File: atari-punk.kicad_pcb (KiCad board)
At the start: 2 copper layers, 74.7 x 54.4 mm, 25 parts, among them J1 Barrel_Jack_Switch, J2 Euro_Power, J3 CV1_IN, J4 CV2_IN, J5 CV3_IN, J6 CV4_IN, J7 AUDIO_OUT, U1 LM555xN, U2 LM555xN

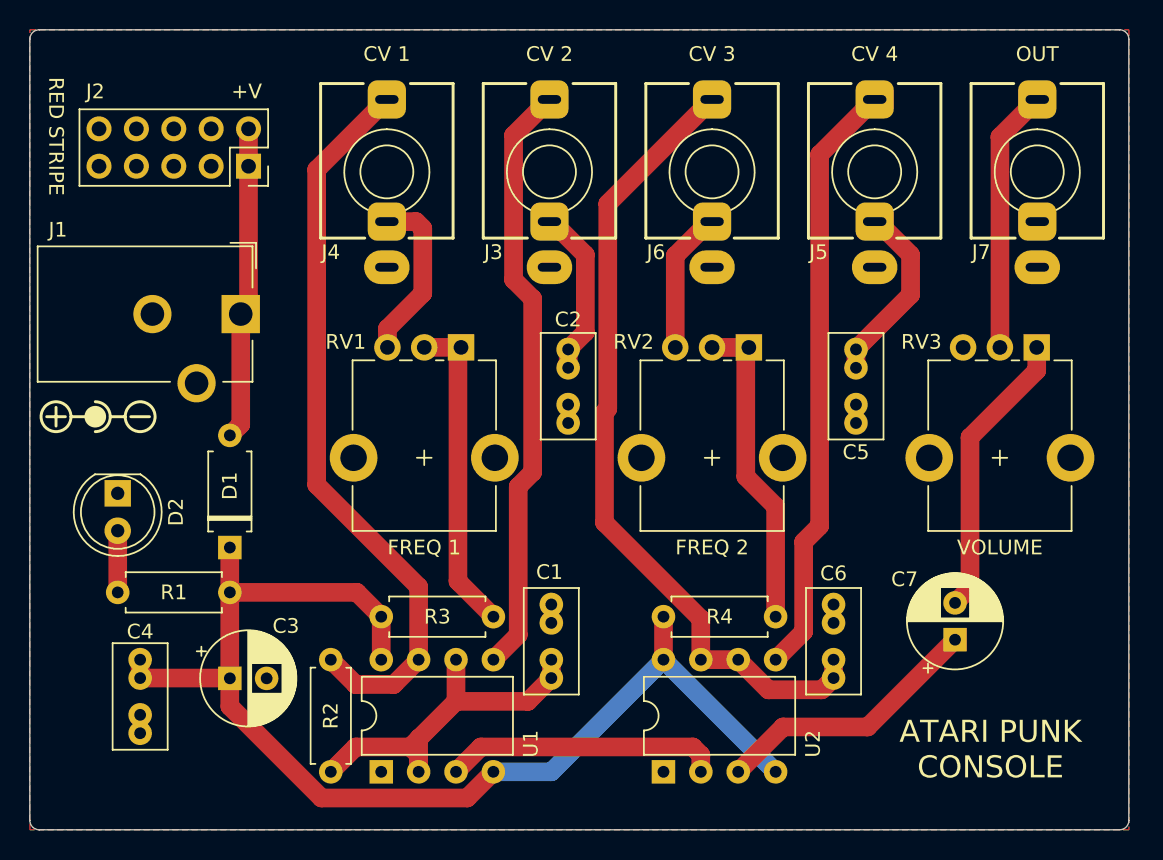
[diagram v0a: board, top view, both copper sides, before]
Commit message: Fixing for rev2
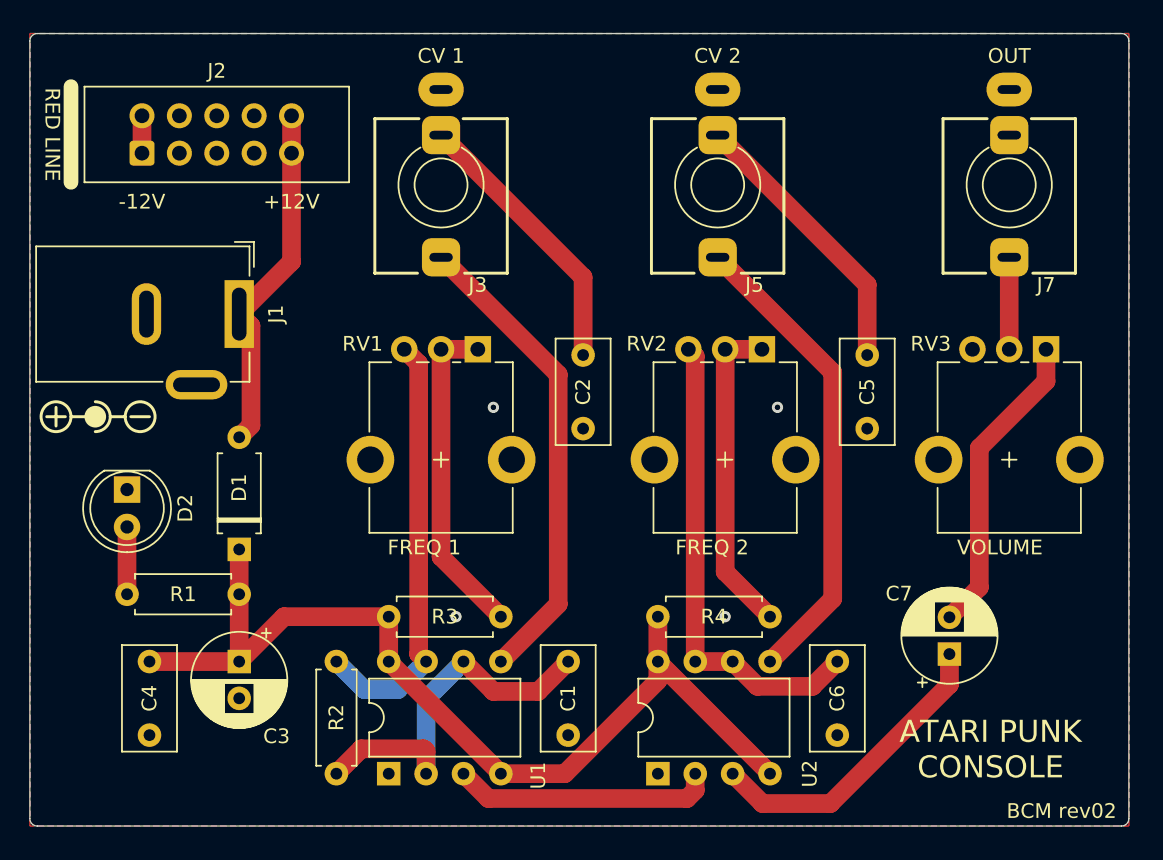
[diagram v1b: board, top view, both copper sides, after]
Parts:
- removed J4: CV2_IN, AudioJacks:Jack_3.5mm_QingPu_WQP-PJ398SM_Vertical
- removed J6: CV4_IN, AudioJacks:Jack_3.5mm_QingPu_WQP-PJ398SM_Vertical
- C1, C2, C4, C5: footprint Rumblesan_Footprints:C_Rect_L7.0mm_W3.5mm_P2.50mm_P5.00mm -> Rumblesan_Footprints:C_Rect_L7.0mm_W3.5mm_P5.00mm
- C6: value 10nF -> 100nF; footprint Rumblesan_Footprints:C_Rect_L7.0mm_W3.5mm_P2.50mm_P5.00mm -> Rumblesan_Footprints:C_Rect_L7.0mm_W3.5mm_P5.00mm
- D1: value 1N5189 -> 1N5818
- J1: footprint Connector_BarrelJack:BarrelJack_CUI_PJ-102AH_Horizontal -> Connector_BarrelJack:BarrelJack_GCT_DCJ200-10-A_Horizontal
- J2: value Euro_Power -> Eurorack_Power_Small; footprint Connector_PinSocket_2.54mm:PinSocket_2x05_P2.54mm_Vertical -> EurorackBasics:Eurorack_PowerHeader_2x05_P2.54mm_Bare
- J3: value CV1_IN -> CV1; footprint AudioJacks:Jack_3.5mm_QingPu_WQP-PJ398SM_Vertical -> EurorackBasics:Jack_3.5mm_QingPu_WQP-PJ398SM_Vertical
- J5: value CV3_IN -> CV2; footprint AudioJacks:Jack_3.5mm_QingPu_WQP-PJ398SM_Vertical -> EurorackBasics:Jack_3.5mm_QingPu_WQP-PJ398SM_Vertical
- J7: footprint AudioJacks:Jack_3.5mm_QingPu_WQP-PJ398SM_Vertical -> EurorackBasics:Jack_3.5mm_QingPu_WQP-PJ398SM_Vertical
- moved J5 10.7 mm to (142.2, 44.8), turned to 180 degrees
- moved J3 7.42 mm to (123.4, 44.8), turned to 180 degrees
- moved J2 7.29 mm to (103.1, 42.7), turned to 90 degrees
- moved J7 2.10 mm to (162.1, 44.8), turned to 180 degrees
- moved C1 1.60 mm to (132.1, 77.2), turned to -90 degrees
- moved C3 1.31 mm to (109.7, 77.2), turned to -90 degrees
- moved C6 1.15 mm to (150.4, 77.2), turned to -90 degrees
- moved RV1 1.15 mm to (123.4, 63.5)
- moved C2 1.09 mm to (133.1, 56.4)
- moved C7 1.05 mm to (158.0, 76.7)
- moved RV2 0.90 mm to (142.7, 63.5)
- moved C5 0.85 mm to (152.4, 56.4)
- moved D2 0.68 mm to (102.1, 65.5)
- moved C4 0.65 mm to (103.6, 77.2)
- moved D1 0.65 mm to (109.7, 69.6)
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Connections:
- J2 pad 1: Net-(D1-Pad2) -> unconnected-(J2-Pad1)
- J2 pad 10: unconnected-(J2-Pad10) -> Net-(D1-Pad2)
- J2 pad 2: Net-(D1-Pad2) -> unconnected-(J2-Pad1)
- J2 pad 9: unconnected-(J2-Pad9) -> Net-(D1-Pad2)
- R2 pad 2: Net-(J4-PadT) -> Net-(R2-Pad2)
- RV1 pad 3: Net-(J4-PadTN) -> Net-(R2-Pad2)
- RV2 pad 3: Net-(J6-PadTN) -> Net-(C6-Pad1)
- U1 pad 7: Net-(J4-PadT) -> Net-(R2-Pad2)
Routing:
- net Net-(J4-PadT): track 50.3 -> 0.00 mm
- net Net-(R2-Pad2): track 0.00 -> 29.5 mm
- net Net-(C6-Pad1): track 55.3 -> 32.5 mm
- net VCC: track 81.7 -> 67.4 mm
- net Net-(J4-PadTN): track 11.7 -> 0.00 mm
- net Net-(J7-PadT): track 17.9 -> 6.25 mm
- net Net-(J6-PadTN): track 9.69 -> 0.00 mm
- net Net-(J5-PadT): track 40.9 -> 32.5 mm
- net Net-(J3-PadT): track 40.7 -> 32.4 mm
- net Net-(C2-Pad1): track 11.5 -> 18.9 mm
- net Net-(C5-Pad1): track 12.6 -> 19.1 mm
- net Net-(D1-Pad2): track 21.4 -> 24.0 mm
- net Net-(C7-Pad1): track 18.5 -> 21.0 mm
- net unconnected-(J2-Pad1): track 0.00 -> 2.54 mm
- net Net-(C7-Pad2): track 19.7 -> 20.9 mm
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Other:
- board size 74.7 x 54.4 mm -> 74.7 x 53.8 mm
- board text added: "BCM rev02"
- board text removed: "+V"
- board text removed: "CV 3"
- board text removed: "CV 4"
- board text removed: "RED STRIPE"

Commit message: Updating layout
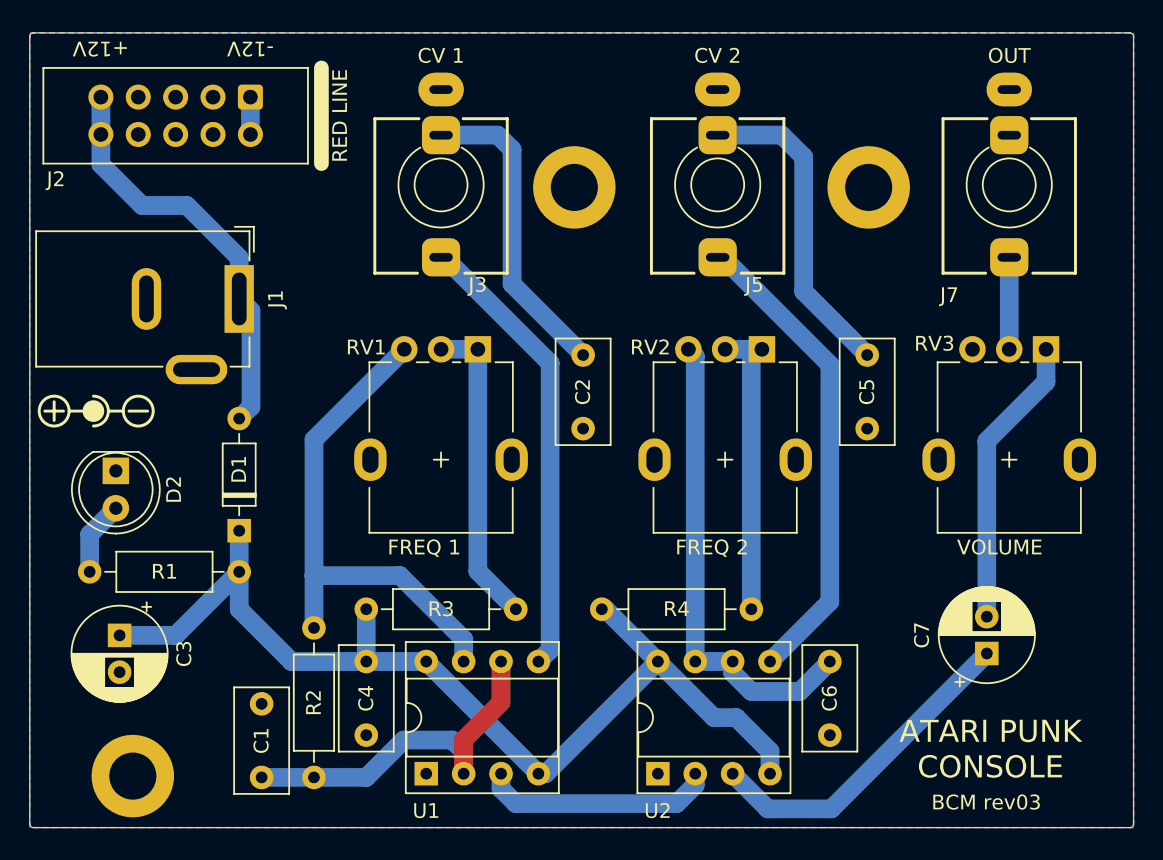
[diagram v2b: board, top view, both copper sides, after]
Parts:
- added H1: MountingHole_Pad, MountingHole:MountingHole_3.2mm_M3_DIN965_Pad, F.Cu at (132.5, 45.0)
- added H2: MountingHole_Pad, MountingHole:MountingHole_3.2mm_M3_DIN965_Pad, F.Cu at (102.5, 85.0)
- added H3: MountingHole_Pad, MountingHole:MountingHole_3.2mm_M3_DIN965_Pad, F.Cu at (152.5, 45.0)
- C1, C2, C4, C5, C6: footprint Rumblesan_Footprints:C_Rect_L7.0mm_W3.5mm_P5.00mm -> rumblesan-standard-parts:C_Rect_L7.0mm_W3.5mm_P5.00mm
- C3, C7: footprint Rumblesan_Footprints:CP_Radial_D6.3mm_P2.50mm -> rumblesan-standard-parts:CP_Radial_D6.3mm_P2.50mm
- D1: footprint Rumblesan_Footprints:Diode_THT_P7.62mm_Horizontal -> rumblesan-standard-parts:D_DO-35_SOD27_P7.62mm_Horizontal
- J2: footprint EurorackBasics:Eurorack_PowerHeader_2x05_P2.54mm_Bare -> eurorack-power:Eurorack_PowerHeader_2x05_P2.54mm_Bare
- J3, J5, J7: footprint EurorackBasics:Jack_3.5mm_QingPu_WQP-PJ398SM_Vertical -> rumblesan-standard-parts:Jack_3.5mm_QingPu_WQP-PJ398SM_Vertical
- R1, R2, R3, R4: footprint Rumblesan_Footprints:R_Axial_DIN0207_L6.3mm_D2.5mm_P7.62mm_Horizontal -> rumblesan-standard-parts:R_Axial_DIN0207_L6.3mm_D2.5mm_P10.16mm_Horizontal
- RV1, RV2, RV3: footprint Rumblesan_Footprints:Potentiometer_Alpha_RD901F-40-00D_Single_Vertical_CircularHoles -> rumblesan-standard-parts:Potentiometer_Alpha_RD901F-40-00D_Single_Vertical
- U1, U2: footprint Package_DIP:DIP-8_W7.62mm -> rumblesan-standard-parts:DIP-8_W7.62mm_Socket
- moved C1 22.3 mm to (111.3, 85.1), turned to 90 degrees
- moved C4 14.7 mm to (118.4, 77.2)
- moved C3 8.32 mm to (101.6, 75.4)
- moved J2 8.29 mm to (110.5, 38.9), turned to -90 degrees
- moved R4 3.84 mm to (134.4, 73.7)
- moved U1 2.55 mm to (122.4, 84.8)
- moved C7 2.54 mm to (160.5, 76.7)
- moved R3 1.61 mm to (118.4, 73.7)
- moved R2 1.55 mm to (114.8, 85.1)
- moved R1 1.52 mm to (109.7, 71.1)
- moved D2 1.48 mm to (101.3, 64.3)
- moved D1 1.27 mm to (109.7, 68.3)
- moved J1 1.03 mm to (109.7, 52.6)
- moved C6 0.51 mm to (149.9, 77.2)
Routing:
- net Net-(R2-Pad2): track 29.5 -> 34.9 mm
- net VCC: track 67.4 -> 72.0 mm
- net Net-(D1-Pad2): track 24.0 -> 28.2 mm
- net Net-(C5-Pad1): track 19.1 -> 21.7 mm
- net Net-(C2-Pad1): track 18.9 -> 21.2 mm
- net Net-(U1-Pad3): track 17.8 -> 15.9 mm
- net Net-(R4-Pad2): track 21.9 -> 20.2 mm
- net Net-(C7-Pad1): track 21.0 -> 22.6 mm
- net Net-(J3-PadT): track 32.4 -> 31.0 mm
- net Net-(R3-Pad2): track 22.4 -> 21.2 mm
- net Net-(C7-Pad2): track 20.9 -> 19.8 mm
- net Net-(C1-Pad1): track 25.9 -> 25.3 mm
- net GND: vias 4 -> 0
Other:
- board size 74.7 x 53.8 mm -> 75 x 54 mm
- board text added: "BCM rev03"
- board text removed: "BCM rev02"
